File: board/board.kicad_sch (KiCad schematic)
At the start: 3 parts, among them J1 001_I2C, J2 011_GPIO

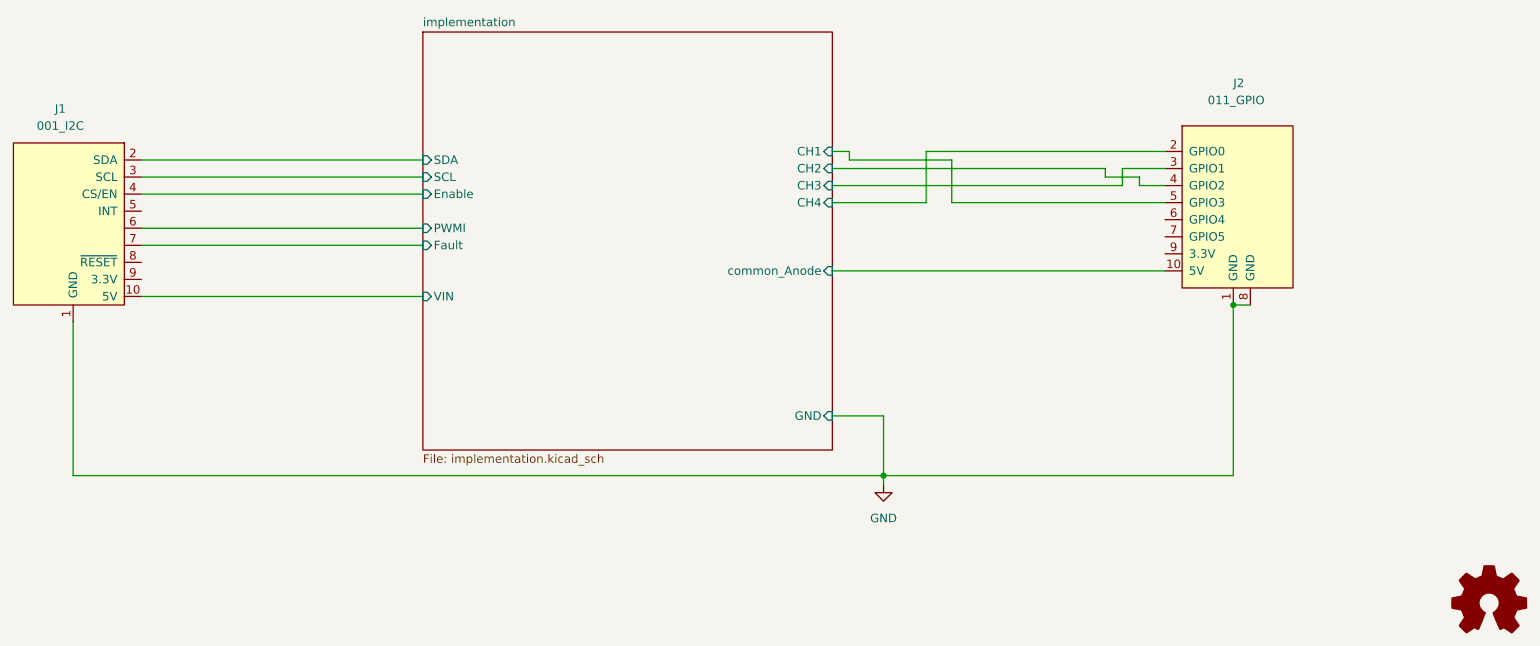
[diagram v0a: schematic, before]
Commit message: Update PCB
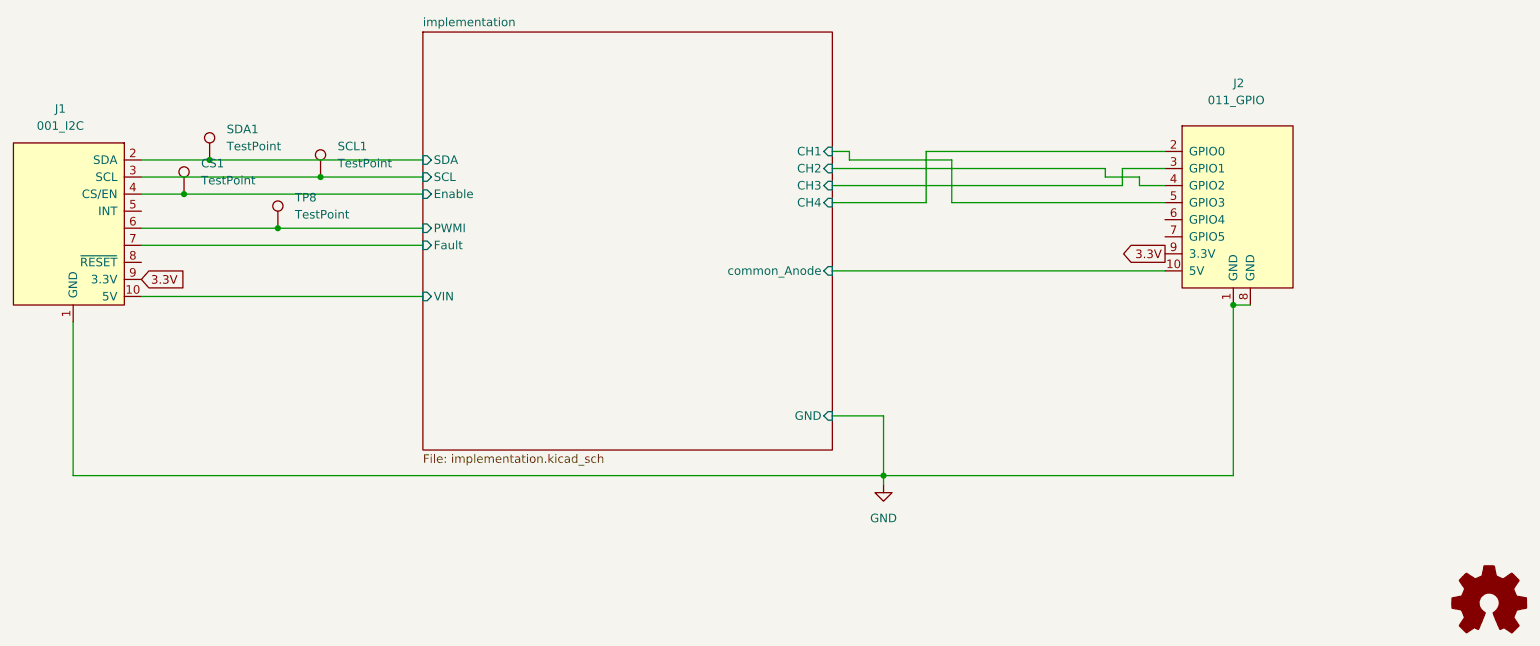
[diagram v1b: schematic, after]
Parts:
- added CS1, SCL1, SDA1, TP8: TestPoint, TestPoint:TestPoint_Pad_D1.0mm, symbol Connector:TestPoint
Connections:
- net implementation/Enable: now also CS1.1
- net implementation/PWMI: now also TP8.1
- net implementation/SCL: now also SCL1.1
- net implementation/SDA: now also SDA1.1
- net 3.3V: now reaches J1.9 (3.3V)
- net 3.3V: now also J2.9 (3.3V)
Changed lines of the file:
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@@
   (junction (at 182.88 138.43) (diameter 0) (color 0 0 0 0)
   )
+  (junction (at 82.55 91.44) (diameter 0) (color 0 0 0 0)
+  )
   (junction (at 234.95 113.03) (diameter 0) (color 0 0 0 0)
   )
+  (junction (at 92.71 101.6) (diameter 0) (color 0 0 0 0)
+  )
+  (junction (at 99.06 93.98) (diameter 0) (color 0 0 0 0)
+  )
+  (junction (at 78.74 96.52) (diameter 0) (color 0 0 0 0)
+  )
   (wire (pts (xy 218.44 95.25) (xy 218.44 92.71))
     (stroke (width 0) (type default))
@@
     (stroke (width 0) (type default))
   )
+  (wire (pts (xy 82.55 91.44) (xy 114.3 91.44))
+    (stroke (width 0) (type default))
+  )
   (wire (pts (xy 193.04 91.44) (xy 177.8 91.44))
     (stroke (width 0) (type default))
   )
-  (wire (pts (xy 72.39 91.44) (xy 114.3 91.44))
+  (wire (pts (xy 99.06 93.98) (xy 114.3 93.98))
+    (stroke (width 0) (type default))
+  )
+  (wire (pts (xy 72.39 91.44) (xy 82.55 91.44))
     (stroke (width 0) (type default))
   )
@@
     (stroke (width 0) (type default))
   )
-  (wire (pts (xy 72.39 101.6) (xy 114.3 101.6))
+  (wire (pts (xy 72.39 101.6) (xy 92.71 101.6))
+    (stroke (width 0) (type default))
+  )
+  (wire (pts (xy 92.71 101.6) (xy 114.3 101.6))
     (stroke (width 0) (type default))
   )
@@
     (stroke (width 0) (type default))
   )
+  (wire (pts (xy 78.74 96.52) (xy 114.3 96.52))
+    (stroke (width 0) (type default))
+  )
   (wire (pts (xy 189.23 90.17) (xy 189.23 97.79))
     (stroke (width 0) (type default))
@@
     (stroke (width 0) (type default))
   )
-  (wire (pts (xy 72.39 93.98) (xy 114.3 93.98))
+  (wire (pts (xy 72.39 93.98) (xy 99.06 93.98))
     (stroke (width 0) (type default))
   )
@@
     (stroke (width 0) (type default))
   )
-  (wire (pts (xy 72.39 96.52) (xy 114.3 96.52))
+  (wire (pts (xy 72.39 96.52) (xy 78.74 96.52))
     (stroke (width 0) (type default))
   )
@@
   (wire (pts (xy 220.98 93.98) (xy 220.98 95.25))
     (stroke (width 0) (type default))
+  )
+  (global_label "3.3V" (shape input) (at 72.39 109.22 0) (fields_autoplaced)
+    (effects (font (size 1.27 1.27)) (justify left))
+    (property "Intersheetrefs" "${INTERSHEET_REFS}" (at 79.4082 109.22 0)
+      (effects (font (size 1.27 1.27)) (justify left) hide)
+    )
+  )
+  (global_label "3.3V" (shape output) (at 224.79 105.41 180) (fields_autoplaced)
+    (effects (font (size 1.27 1.27)) (justify right))
+    (property "Intersheetrefs" "${INTERSHEET_REFS}" (at 217.7718 105.41 0)
+      (effects (font (size 1.27 1.27)) (justify right) hide)
+    )
   )
   (symbol (lib_id "put_on_edge:001_I2C") (at 60.96 101.6 0) (mirror y) (unit 1)
@@
     )
   )
+  (symbol (lib_id "Connector:TestPoint") (at 92.71 101.6 0) (unit 1)
+    (in_bom yes) (on_board yes) (dnp no) (fields_autoplaced)
+    (property "Reference" "TP8" (at 95.25 97.028 0)
+      (effects (font (size 1.27 1.27)) (justify left))
+    )
+    (property "Value" "TestPoint" (at 95.25 99.568 0)
+      (effects (font (size 1.27 1.27)) (justify left))
+    )
+    (property "Footprint" "TestPoint:TestPoint_Pad_D1.0mm" (at 97.79 101.6 0)
+      (effects (font (size 1.27 1.27)) hide)
+    )
+    (property "Datasheet" "~" (at 97.79 101.6 0)
+      (effects (font (size 1.27 1.27)) hide)
+    )
+    (pin "1")
+    (instances
+      (project "board"
+        (path "/57732dd3-1162-4c3f-88bd-31bf473d124d/767ce4c6-0e55-4543-92f0-34cb8237a544"
+          (reference "TP8") (unit 1)
+        )
+        (path "/57732dd3-1162-4c3f-88bd-31bf473d124d"
+          (reference "PWMI1") (unit 1)
+        )
+      )
+    )
+  )
+  (symbol (lib_id "Connector:TestPoint") (at 78.74 96.52 0) (unit 1)
+    (in_bom yes) (on_board yes) (dnp no) (fields_autoplaced)
+    (property "Reference" "CS1" (at 81.28 91.948 0)
+      (effects (font (size 1.27 1.27)) (justify left))
+    )
+    (property "Value" "TestPoint" (at 81.28 94.488 0)
+      (effects (font (size 1.27 1.27)) (justify left))
+    )
+    (property "Footprint" "TestPoint:TestPoint_Pad_D1.0mm" (at 83.82 96.52 0)
+      (effects (font (size 1.27 1.27)) hide)
+    )
+    (property "Datasheet" "~" (at 83.82 96.52 0)
+      (effects (font (size 1.27 1.27)) hide)
+    )
+    (pin "1")
+    (instances
+      (project "board"
+        (path "/57732dd3-1162-4c3f-88bd-31bf473d124d"
+          (reference "CS1") (unit 1)
+        )
+      )
+    )
+  )
   (symbol (lib_id "put_on_edge:011_GPIO") (at 236.22 99.06 0) (unit 1)
     (in_bom yes) (on_board yes) (dnp no)
@@
         )
       )
+    )
+  )
+  (symbol (lib_id "Connector:TestPoint") (at 82.55 91.44 0) (unit 1)
+    (in_bom yes) (on_board yes) (dnp no) (fields_autoplaced)
+    (property "Reference" "SDA1" (at 85.09 86.868 0)
+      (effects (font (size 1.27 1.27)) (justify left))
+    )
+    (property "Value" "TestPoint" (at 85.09 89.408 0)
+      (effects (font (size 1.27 1.27)) (justify left))
+    )
+    (property "Footprint" "TestPoint:TestPoint_Pad_D1.0mm" (at 87.63 91.44 0)
+      (effects (font (size 1.27 1.27)) hide)
+    )
+    (property "Datasheet" "~" (at 87.63 91.44 0)
+      (effects (font (size 1.27 1.27)) hide)
+    )
+    (pin "1")
+    (instances
+      (project "board"
+        (path "/57732dd3-1162-4c3f-88bd-31bf473d124d"
+          (reference "SDA1") (unit 1)
+        )
+      )
+    )
+  )
+  (symbol (lib_id "Connector:TestPoint") (at 99.06 93.98 0) (unit 1)
+    (in_bom yes) (on_board yes) (dnp no) (fields_autoplaced)
+    (property "Reference" "SCL1" (at 101.6 89.408 0)
+      (effects (font (size 1.27 1.27)) (justify left))
+    )
+    (property "Value" "TestPoint" (at 101.6 91.948 0)
+      (effects (font (size 1.27 1.27)) (justify left))
+    )
+    (property "Footprint" "TestPoint:TestPoint_Pad_D1.0mm" (at 104.14 93.98 0)
+      (effects (font (size 1.27 1.27)) hide)
+    )
+    (property "Datasheet" "~" (at 104.14 93.98 0)
+      (effects (font (size 1.27 1.27)) hide)
+    )
+    (pin "1")
+    (instances
+      (project "board"
+        (path "/57732dd3-1162-4c3f-88bd-31bf473d124d"
+          (reference "SCL1") (unit 1)
+        )
+      )
